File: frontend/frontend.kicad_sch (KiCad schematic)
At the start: 148 parts, among them J1 REF_IN, J10 GND, J11 Conn_02x13_Odd_Even, J12 Conn_01x01_Socket, J14 Conn_01x01_Socket, J15 Conn_01x01_Socket, J16 Conn_01x01_Socket, J17 Conn_01x01_Socket, J19 A, J2 REF_S_P, J3 REF_S_N, J4 REF_GND, J5 mA, J6 V, J7 Common, J8 +6V, J9 -10V, K1 NRP26-A05D, K2 NRP26-A05D, Q2 MMBT2222A, Q3 MMBT2222A, U1 ADG722, U12 MAX4208, U13 OPA2186DR, U14 ADG722, U16 ADG722, U2 ADG722, U3 OPA2186DR, U4 LM358, U5 LTC2508CDKD-32, U6 ADG722, U8 TCA9535DBR

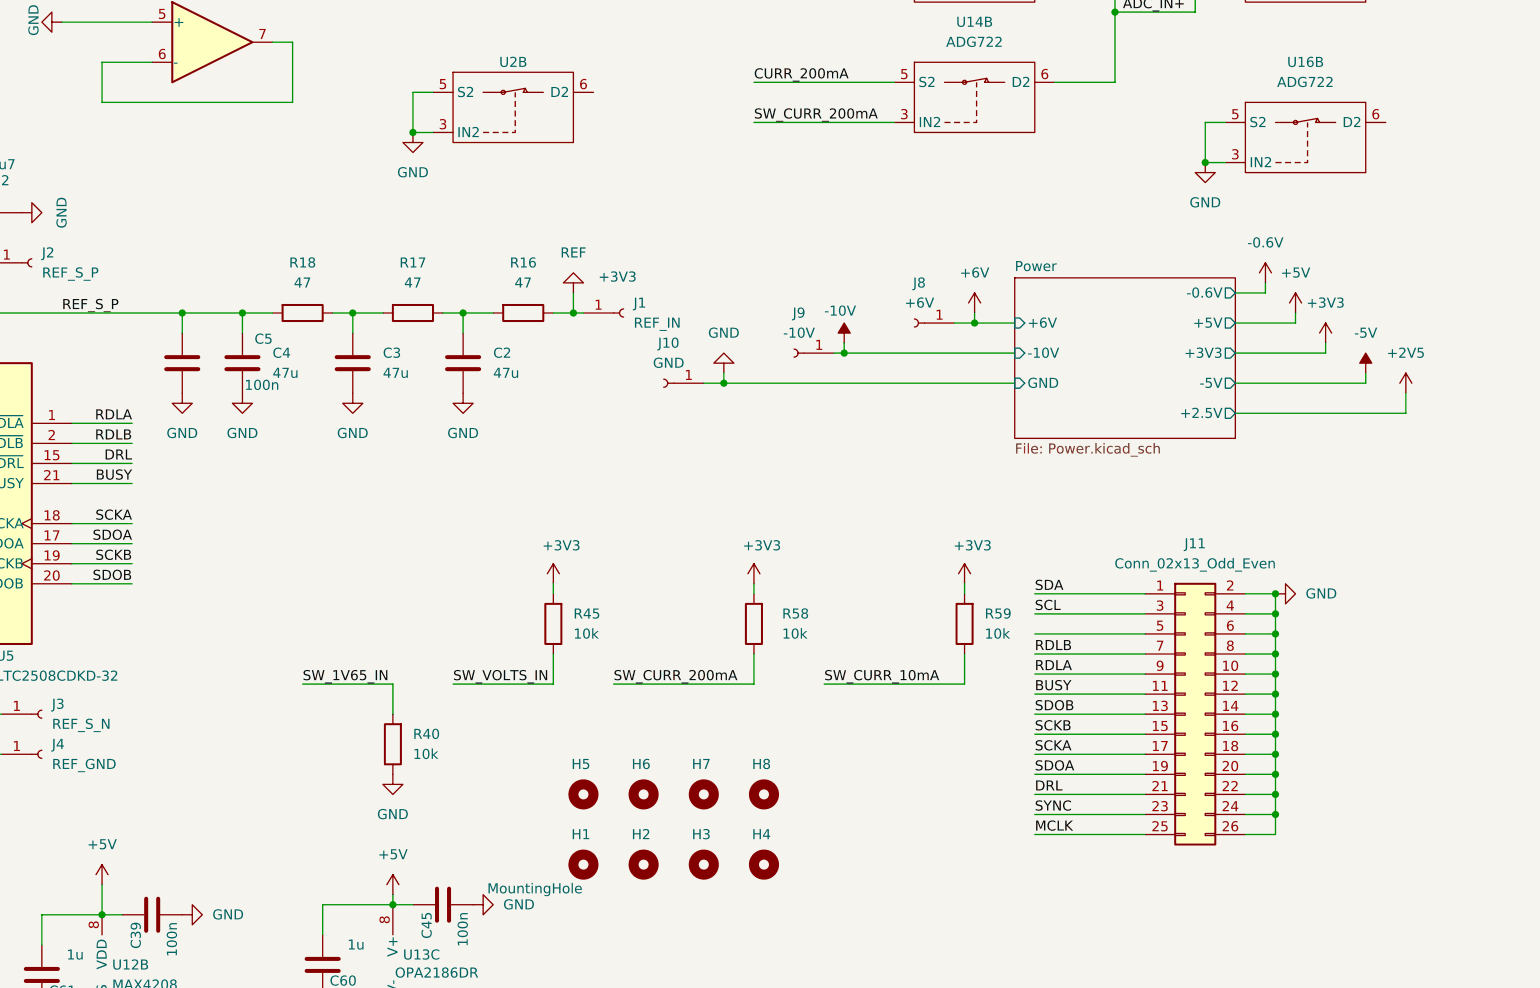
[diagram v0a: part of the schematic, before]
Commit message: 14
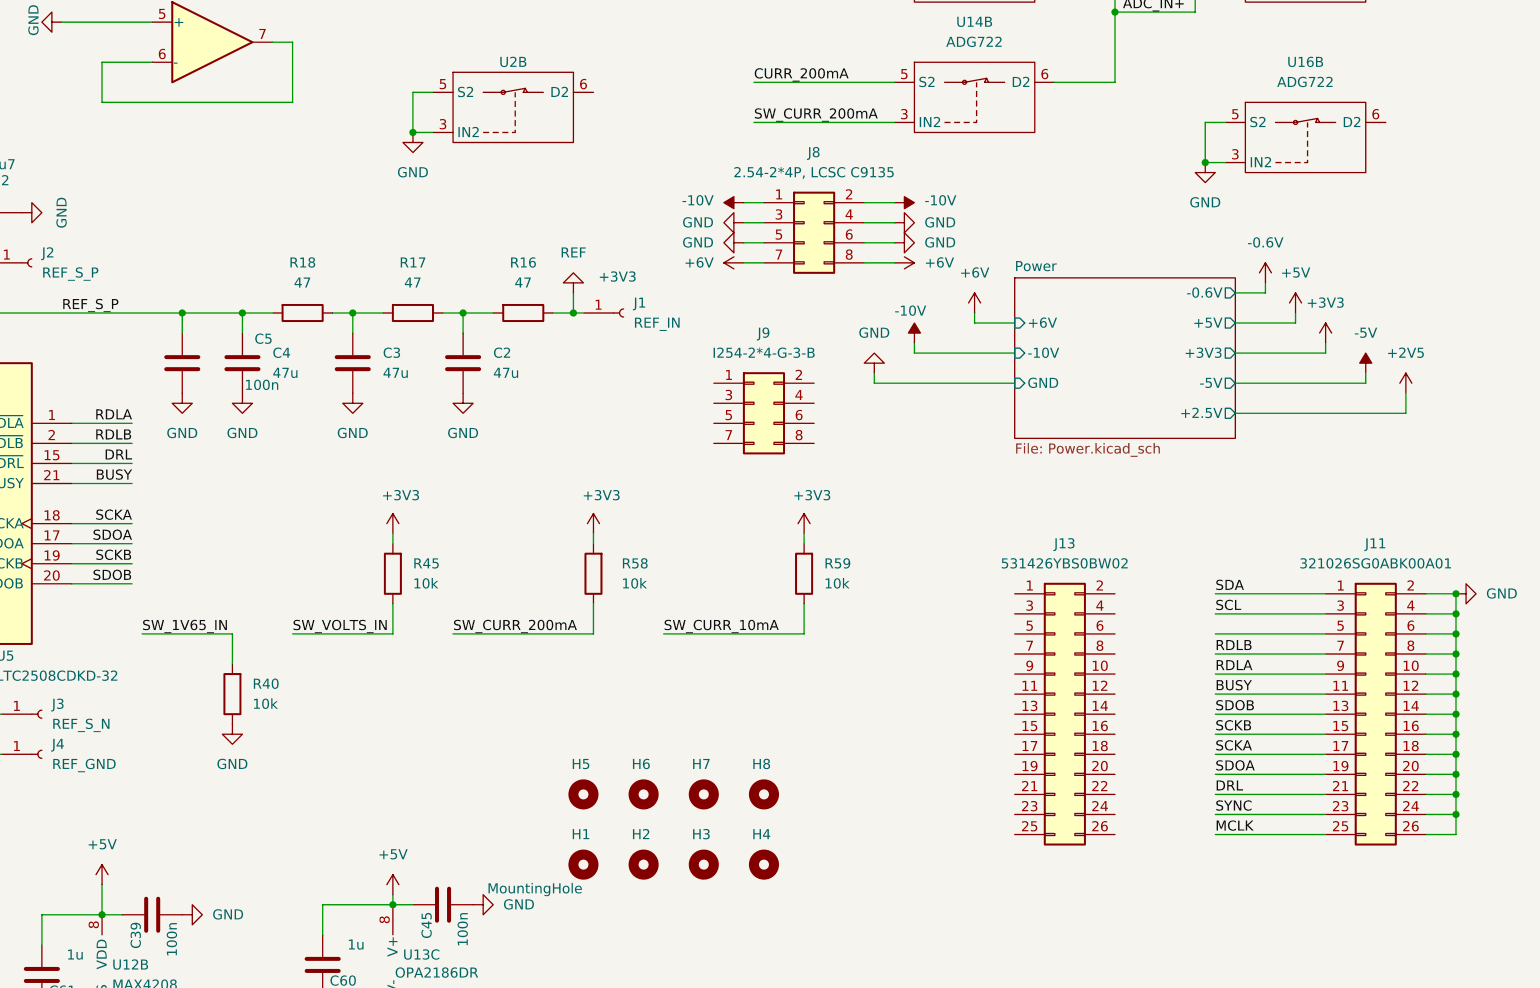
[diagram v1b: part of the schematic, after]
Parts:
- removed J10: GND, Passives:Conn-1-6x6-OD3mm, symbol Connector:Conn_01x01_Socket
- removed J8: +6V, Passives:Conn-1-6x6-OD3mm, symbol Connector:Conn_01x01_Socket
- removed J9: -10V, Passives:Conn-1-6x6-OD3mm, symbol Connector:Conn_01x01_Socket
- added J13: 531426YBS0BW02, Connector_IDC:IDC-Header_2x13_P2.54mm_Vertical, symbol Connector_Generic:Conn_02x13_Odd_Even
- added J8: 2.54-2*4P, LCSC C9135, Connector_IDC:IDC-Header_2x04_P2.54mm_Vertical, symbol Connector_Generic:Conn_02x04_Odd_Even
- added J9: I254-2*4-G-3-B, Connector_IDC:IDC-Header_2x04_P2.54mm_Vertical, symbol Connector_Generic:Conn_02x04_Odd_Even
- J11: value Conn_02x13_Odd_Even -> 321026SG0ABK00A01
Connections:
- net +6V: now also J8.7 (Pin_7), J8.8 (Pin_8)
- net -10V: now also J8.1 (Pin_1), J8.2 (Pin_2)
- net GND: now also J8.3 (Pin_3), J8.4 (Pin_4), J8.5 (Pin_5), J8.6 (Pin_6)
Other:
- moved on the sheet: J11, R40, R45, R58, R59
